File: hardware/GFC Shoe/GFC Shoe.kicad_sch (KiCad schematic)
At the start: 15 parts

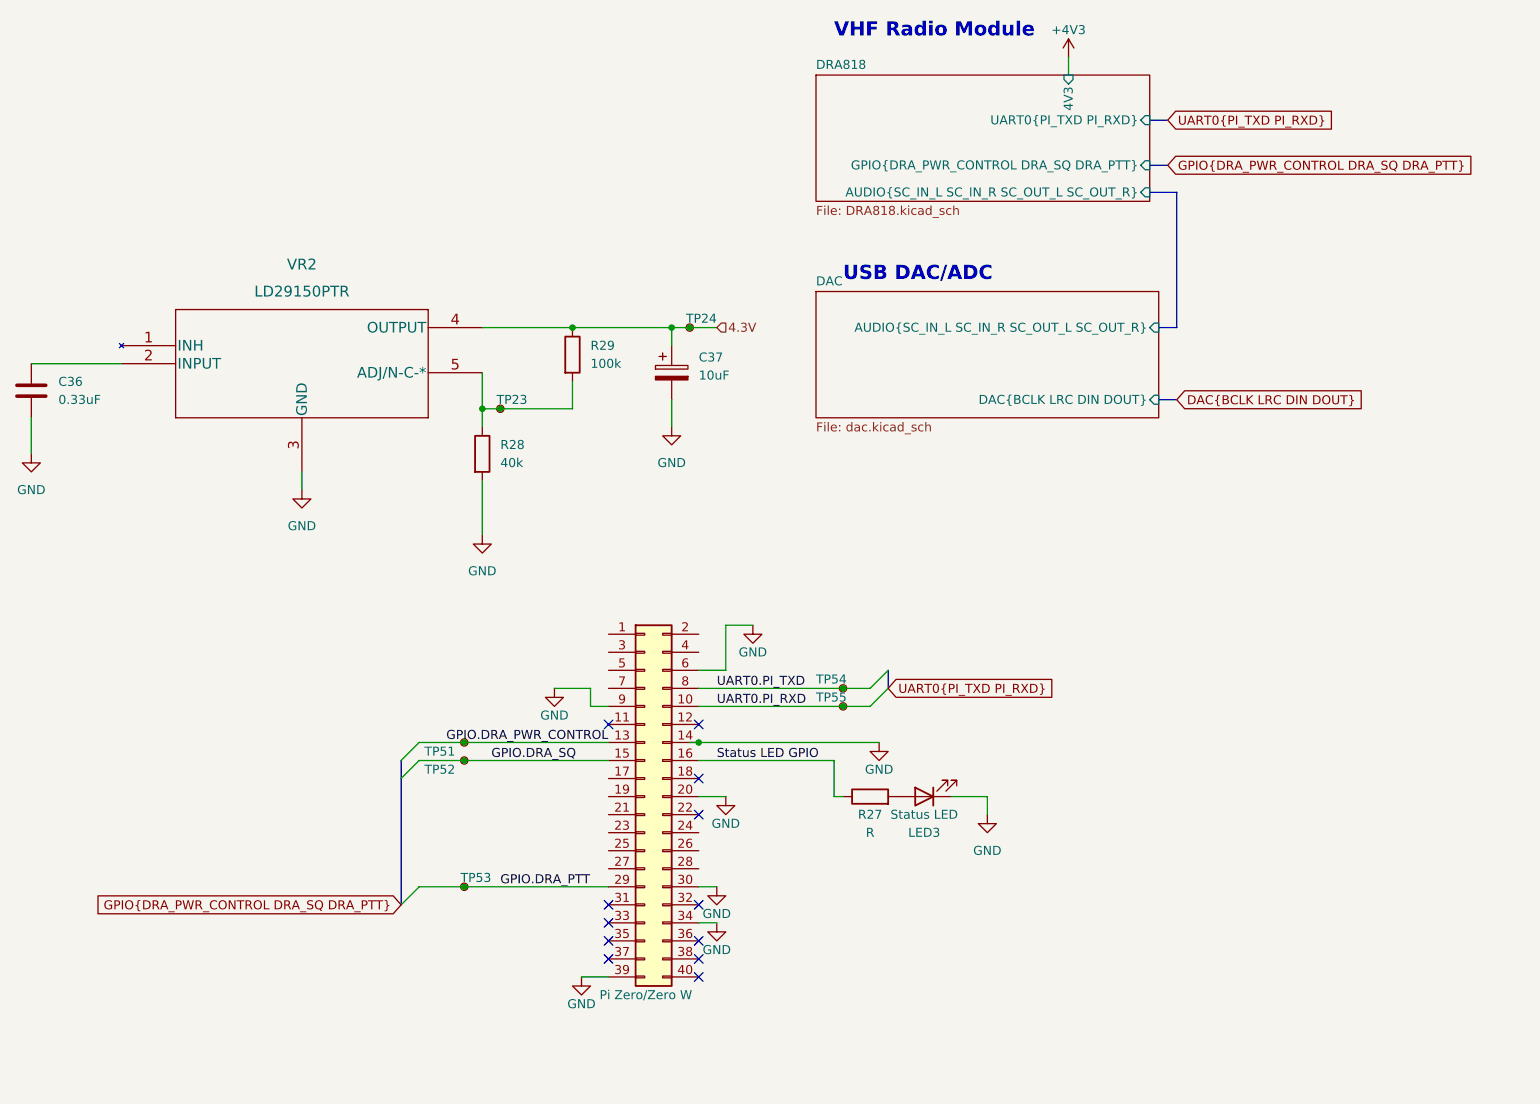
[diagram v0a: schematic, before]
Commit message: Radio/Sound Card PCB Update
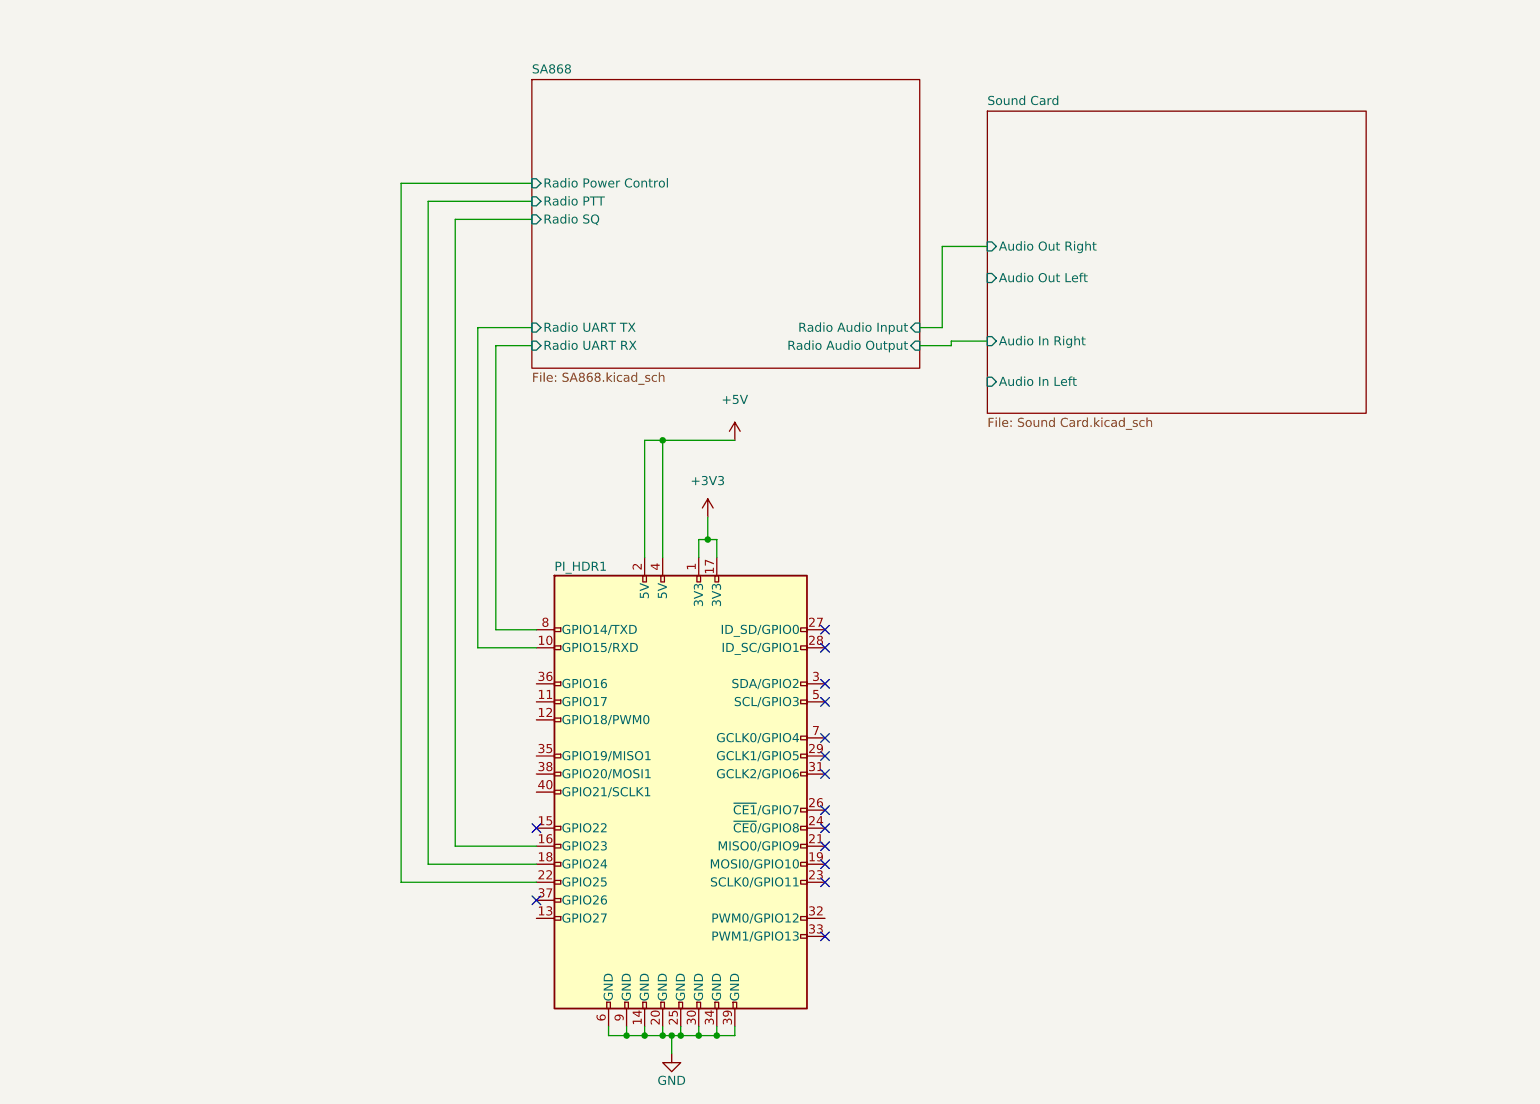
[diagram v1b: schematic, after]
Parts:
- removed C36: 0.33uF, Capacitor_SMD:C_0603_1608Metric_Pad1.08x0.95mm_HandSolder, symbol Device:C
- removed C37: 10uF, Capacitor_SMD:C_0805_2012Metric_Pad1.18x1.45mm_HandSolder, symbol Device:C_Polarized
- removed CPU3: Pi Zero/Zero W, Connector_PinSocket_2.54mm:PinSocket_2x20_P2.54mm_Vertical, symbol Connector_Generic:Conn_02x20_Odd_Even
- removed LED3: Status LED, LED_SMD:LED_0805_2012Metric, symbol Device:LED
- removed R27: R, Resistor_SMD:R_0603_1608Metric_Pad0.98x0.95mm_HandSolder, symbol Device:R
- removed R28: 40k, Resistor_SMD:R_0603_1608Metric_Pad0.98x0.95mm_HandSolder, symbol Device:R
- removed R29: 100k, Resistor_SMD:R_0603_1608Metric_Pad0.98x0.95mm_HandSolder, symbol Device:R
- removed TP23, TP24, TP51, TP52, TP53, TP54, TP55: Test Point, TestPoint:TestPoint_Pad_D1.0mm, symbol Connector:TestPoint_Small
- removed VR2: LD29150PTR, footprints:LD29150PTR, symbol LDV VReg:LD29150PTR
- added PI_HDR1: PI, Connector_PinSocket_2.54mm:PinSocket_2x20_P2.54mm_Vertical, symbol Connector:Raspberry_Pi_2_3
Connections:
- net GND: now also PI_HDR1.14 (GND), PI_HDR1.20 (GND), PI_HDR1.25 (GND), PI_HDR1.30 (GND), PI_HDR1.34 (GND), PI_HDR1.39 (GND), PI_HDR1.6 (GND), PI_HDR1.9 (GND)
- new net +3V3: PI_HDR1.1 (3V3), PI_HDR1.17 (3V3)
- new net +5V: PI_HDR1.2 (5V), PI_HDR1.4 (5V)
- new net SA868/Radio PTT: PI_HDR1.18 (GPIO24)
- new net SA868/Radio Power Control: PI_HDR1.22 (GPIO25)
- new net SA868/Radio SQ: PI_HDR1.16 (GPIO23)
- new net SA868/Radio UART RX: PI_HDR1.8 (GPIO14/TXD)
- new net SA868/Radio UART TX: PI_HDR1.10 (GPIO15/RXD)
- no-connect marks 12 -> 15
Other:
- removed sheet DAC
- removed sheet DRA818
- added sheet SA868 (SA868.kicad_sch)
- added sheet Sound Card (Sound Card.kicad_sch)
- note removed: "USB DAC/ADC"
- note removed: "VHF Radio Module"
